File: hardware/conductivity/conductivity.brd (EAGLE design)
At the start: 32.4 x 31.4 mm, 19 parts, among them IC1 AD820R, U1 TLV2374IDR, U2 TLE2426CD

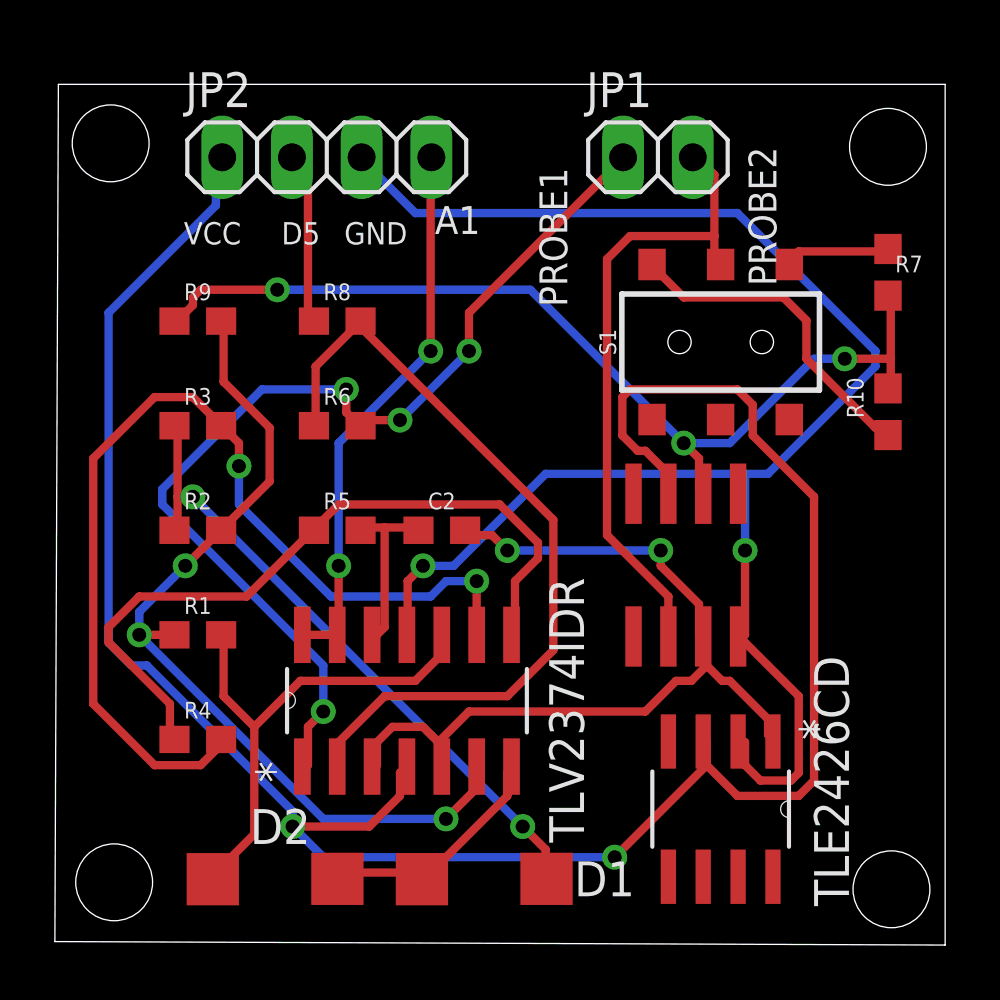
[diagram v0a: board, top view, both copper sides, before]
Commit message: Revert "Updating."
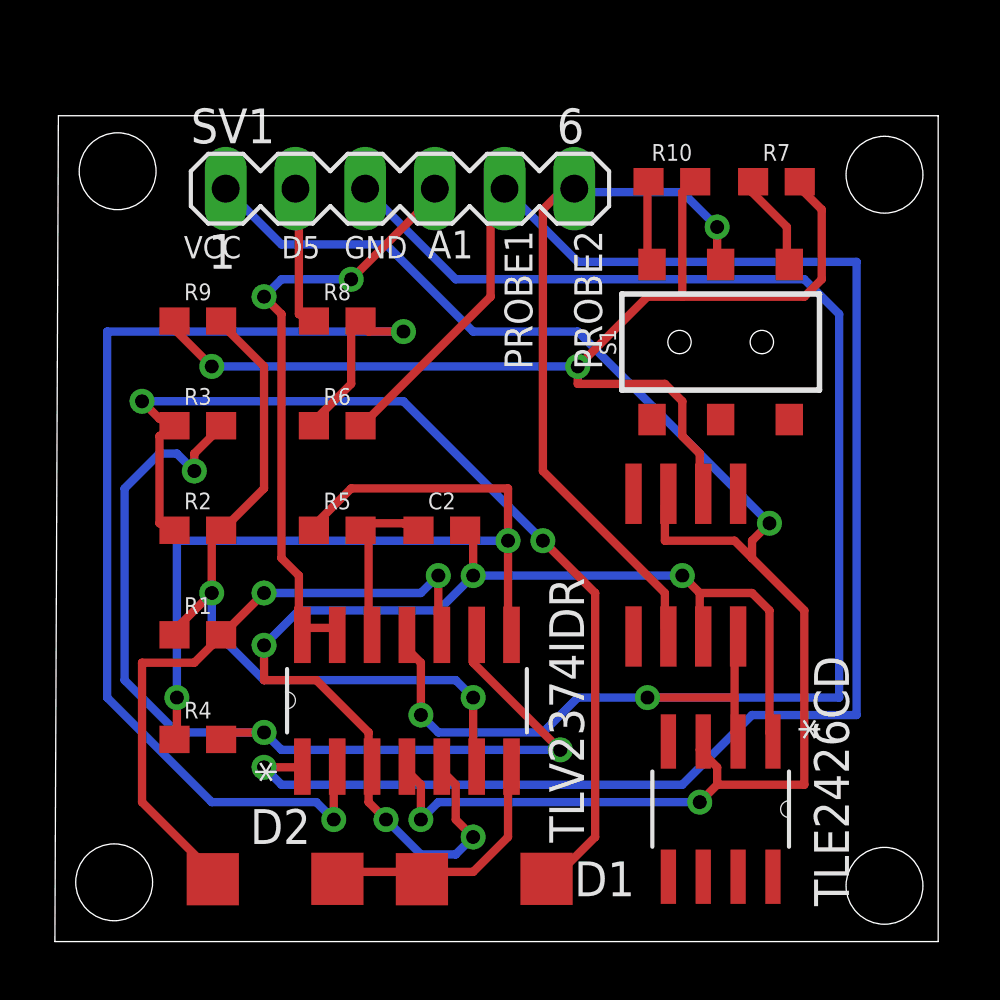
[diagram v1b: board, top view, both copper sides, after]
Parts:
- removed JP1: (no value), pinhead:1X02
- removed JP2: (no value), pinhead:1X04
- added SV1: (no value), con-lstb:MA06-1
- moved R10 11.5 mm to (22.5, 27.7), turned to 0 degrees
- moved R7 5.24 mm to (26.3, 27.7), turned to 0 degrees
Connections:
- net FROMWATER: now also SV1.6; no longer JP1.2
- net N$1: now also SV1.1; no longer JP2.1
- net N$13: now also SV1.4; no longer JP2.4
- net N$14: now also SV1.2; no longer JP2.2
- net N$15: now also SV1.3; no longer JP2.3
- net N$16: now also SV1.5; no longer JP1.1
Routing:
- net N$16: track 37.2 -> 65.8 mm, vias 4 -> 1
- net N$1: track 82.3 -> 59.3 mm, vias 2 -> 3
- net N$4: track 29.5 -> 42.5 mm, vias 0 -> 2
- net N$7: track 23.7 -> 36.6 mm
- net N$3: track 33.9 -> 44.7 mm, vias 2 -> 5
- net N$2: track 12.0 -> 3.12 mm
- net N$5: track 35.9 -> 42.4 mm, vias 3 -> 2
- net N$11: track 27.0 -> 32.5 mm, vias 0 -> 2
- net N$9: track 18.8 -> 23.2 mm, vias 0 -> 2
- net N$6: track 31.7 -> 27.8 mm, vias 3 -> 2
- net FROMWATER: track 23.3 -> 26.1 mm, vias 0 -> 1
- net N$13: track 20.1 -> 22.6 mm
- net N$14: track 6.40 -> 5.23 mm
- net N$8: track 8.88 -> 9.76 mm
- net N$15: track 59.9 -> 59.4 mm
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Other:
- board size 32.4 x 31.4 mm -> 32.2 x 30.1 mm
- board text added: "06/12/19"
- board text removed: "10/18/19"

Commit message: november update
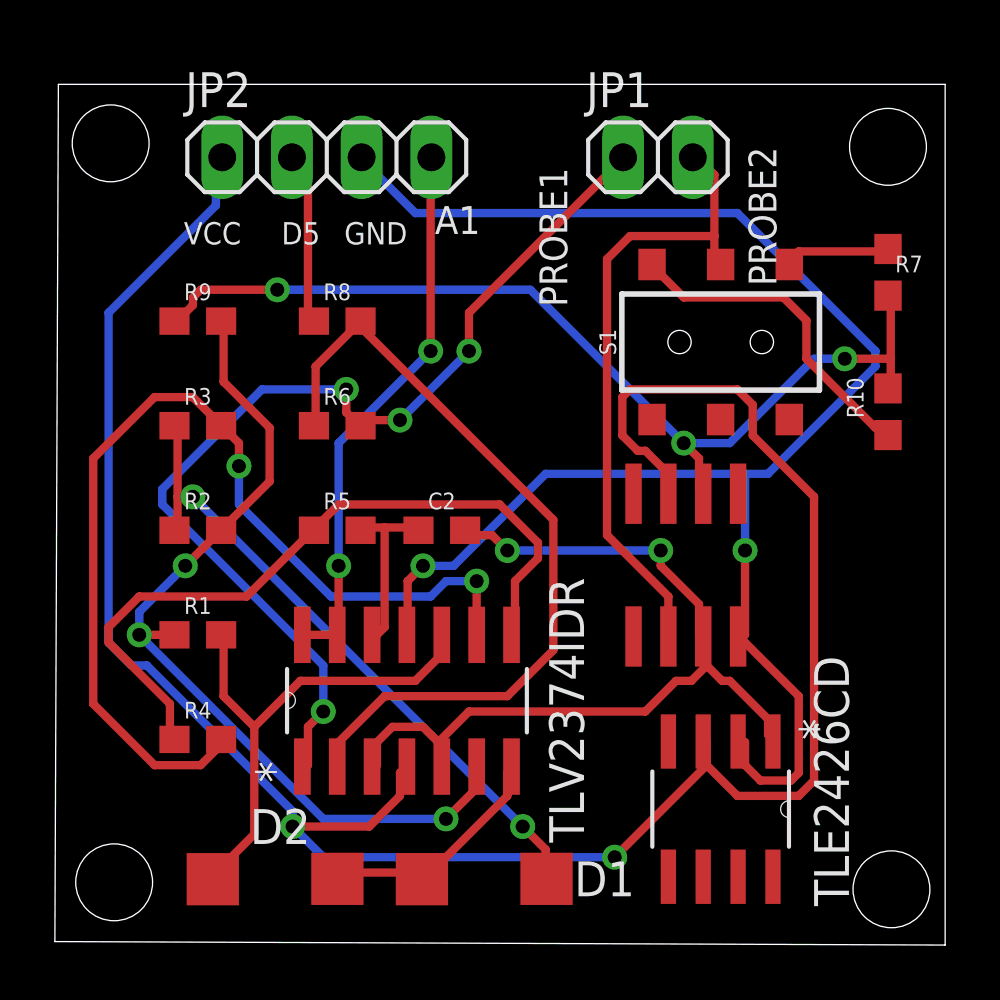
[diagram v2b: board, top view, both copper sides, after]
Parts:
- removed SV1: (no value), con-lstb:MA06-1
- added JP1: (no value), pinhead:1X02
- added JP2: (no value), pinhead:1X04
- moved R10 11.5 mm to (30.4, 19.3), turned to 90 degrees
- moved R7 5.24 mm to (30.4, 24.4), turned to 270 degrees
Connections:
- net FROMWATER: now also JP1.2; no longer SV1.6
- net N$1: now also JP2.1; no longer SV1.1
- net N$13: now also JP2.4; no longer SV1.4
- net N$14: now also JP2.2; no longer SV1.2
- net N$15: now also JP2.3; no longer SV1.3
- net N$16: now also JP1.1; no longer SV1.5
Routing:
- net N$16: track 65.8 -> 37.2 mm, vias 1 -> 4
- net N$1: track 59.3 -> 82.3 mm, vias 3 -> 2
- net N$4: track 42.5 -> 29.5 mm, vias 2 -> 0
- net N$7: track 36.6 -> 23.7 mm
- net N$3: track 44.7 -> 33.9 mm, vias 5 -> 2
- net N$2: track 3.12 -> 12.0 mm
- net N$5: track 42.4 -> 35.9 mm, vias 2 -> 3
- net N$11: track 32.5 -> 27.0 mm, vias 2 -> 0
- net N$9: track 23.2 -> 18.8 mm, vias 2 -> 0
- net N$6: track 27.8 -> 31.7 mm, vias 2 -> 3
- net FROMWATER: track 26.1 -> 23.3 mm, vias 1 -> 0
- net N$13: track 22.6 -> 20.1 mm
- net N$14: track 5.23 -> 6.40 mm
- net N$8: track 9.76 -> 8.88 mm
- net N$15: track 59.4 -> 59.9 mm
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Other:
- board size 32.2 x 30.1 mm -> 32.4 x 31.4 mm
- board text added: "10/18/19"
- board text removed: "06/12/19"
